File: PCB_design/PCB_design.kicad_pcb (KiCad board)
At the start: 2 copper layers, 59.7 x 59.7 mm, 48 parts, among them J10 Conn_01x01_Socket, J11 Conn_01x01_Socket, J2 Conn_01x04_Socket, J3 Conn_01x01_Socket, J4 Conn_01x02_Pin, J5 Conn_01x01_Socket, J6 Conn_01x01_Socket, J7 Conn_01x01_Socket, J8 Conn_01x01_Socket, J9 USB_C_Receptacle_PowerOnly_6P, Q1 FS8205A, U1 L298N, U2 L7805, U3 TP4056, U4 DW01A

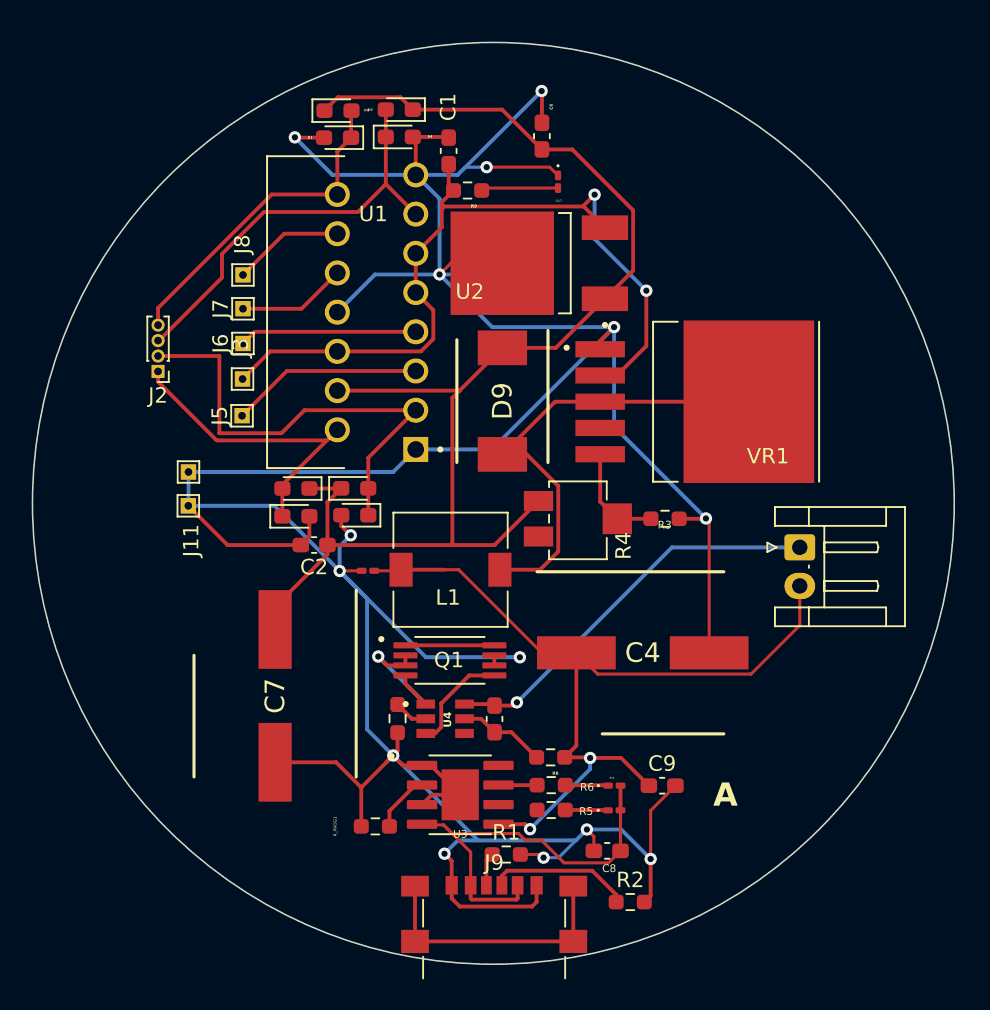
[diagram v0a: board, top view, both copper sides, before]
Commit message: Add new PCB Design
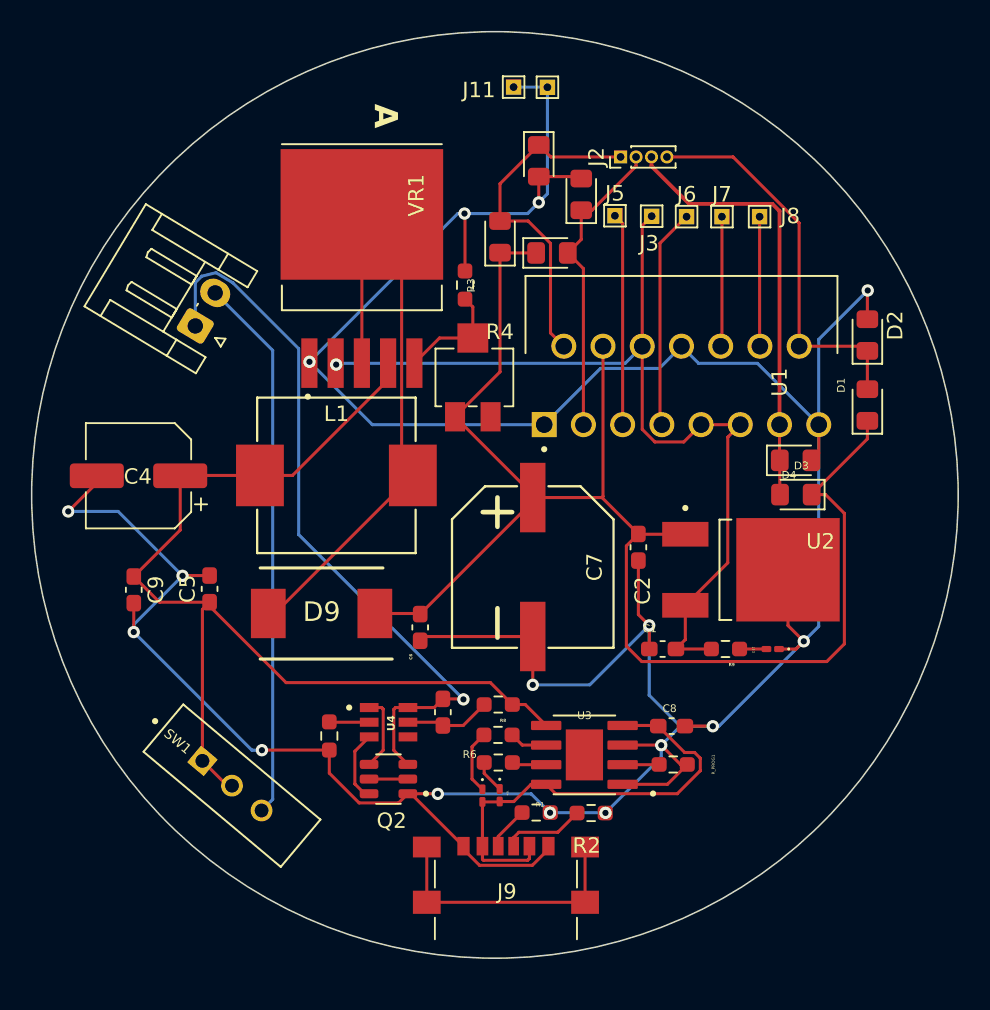
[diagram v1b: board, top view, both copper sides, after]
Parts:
- removed Q1: FS8205A, FS8205A:SOP65P640X120-8N
- added Q2: FS8205, FS8205:SOT95P280X145-6N, F.Cu at (95.3, 82.9)
- added SW1: SW_SPDT, MINI-SPDT-SW:SW_MINI-SPDT-SW, F.Cu at (85.1, 83.3)
- C4: footprint Capacitor_220uF35V_smaller:CAPAE1050X1050N -> Capacitor_SMD:CP_Elec_6.3x7.7
- C5: footprint Capacitor_SMD:C_0201_0603Metric_Pad0.64x0.40mm_HandSolder -> Capacitor_SMD:C_0603_1608Metric_Pad1.08x0.95mm_HandSolder
- C7: footprint Capacitor_220uF35V_smaller:CAPAE1050X1050N -> CAP-SMD_BD10.0-L10.3-W10.3-FD:CAP-SMD_BD10.0-L10.3-W10.3-FD
- D1, D2, D3, D4, D5, D6, D7, D8: footprint Diode_SMD:D_0603_1608Metric_Pad1.05x0.95mm_HandSolder -> Diode_SMD:D_0805_2012Metric_Pad1.15x1.40mm_HandSolder
- L1: footprint Inductor_SMD:L_7.3x7.3_H3.5 -> Inductor_SMD:ND-SMD_L11.6-W10.1_final_13mm
- moved J4 41.7 mm to (82.8, 53.5), turned to 59 degrees
- moved D1 39.2 mm to (126.3, 58.7), turned to 90 degrees
- moved D2 36.6 mm to (126.3, 54.1), turned to 90 degrees
- moved C9 36.5 mm to (78.8, 70.6), turned to -90 degrees
- moved D3 35.8 mm to (121.6, 64.5)
- moved C1 35.1 mm to (113.0, 74.5), turned to 180 degrees
- moved C4 34.6 mm to (79.1, 63.2), turned to 180 degrees
- moved J11 34.3 mm to (103.4, 38.1), turned to 180 degrees
- moved J10 34.1 mm to (105.6, 38.1), turned to 180 degrees
- moved R9 34.1 mm to (117.1, 74.5)
- moved J8 33.7 mm to (119.3, 46.5), turned to 0 degrees
- moved D17 33.3 mm to (120.2, 74.5), turned to 180 degrees
- moved D4 33.1 mm to (121.6, 62.2)
- moved J2 33.0 mm to (110.3, 42.6), turned to 90 degrees
- moved C6 32.8 mm to (97.3, 73.1), turned to -90 degrees
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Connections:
- J4 pad 2: Bat+ -> Net-(J4-Pin_2)
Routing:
- net Net-(J4-Pin_2): track 0.00 -> 35.4 mm
- net Batt-: track 32.8 -> 47.5 mm, vias 2 -> 1
- net Bat+: track 57.1 -> 68.8 mm, vias 2 -> 0
- net Net-(D9-B): track 30.3 -> 41.0 mm
- net GND_Arduino1: track 253.9 -> 243.3 mm, vias 14 -> 16
- net OUT2: track 30.4 -> 20.0 mm
- net Boost_Out: track 87.9 -> 95.6 mm
- net +5V Arduino: track 53.8 -> 60.2 mm, vias 2 -> 1
- net Net-(Q1-Pad1): track 5.76 -> 0.00 mm
- net Net-(J9-CC2): track 9.27 -> 5.32 mm
- net OUT4: track 21.5 -> 25.3 mm
- net Net-(D17-A): track 5.02 -> 1.74 mm
- net A1: track 11.5 -> 14.2 mm
- net Net-(Q2-Pad2): track 0.00 -> 2.51 mm
- net Net-(U4-OD): track 2.40 -> 4.91 mm
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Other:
- board size 59.7 x 59.7 mm -> 60 x 60 mm
